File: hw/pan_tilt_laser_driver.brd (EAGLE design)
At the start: 76.2 x 34.2 mm, 38 parts, among them IC5 93C46, J1 POWER_JACKPTH, U1 CAT6219-330TDGT3, U3 LD3985M30R, X1 798-ZX62RD-AB-5P8, Y1 405I35D12M00000

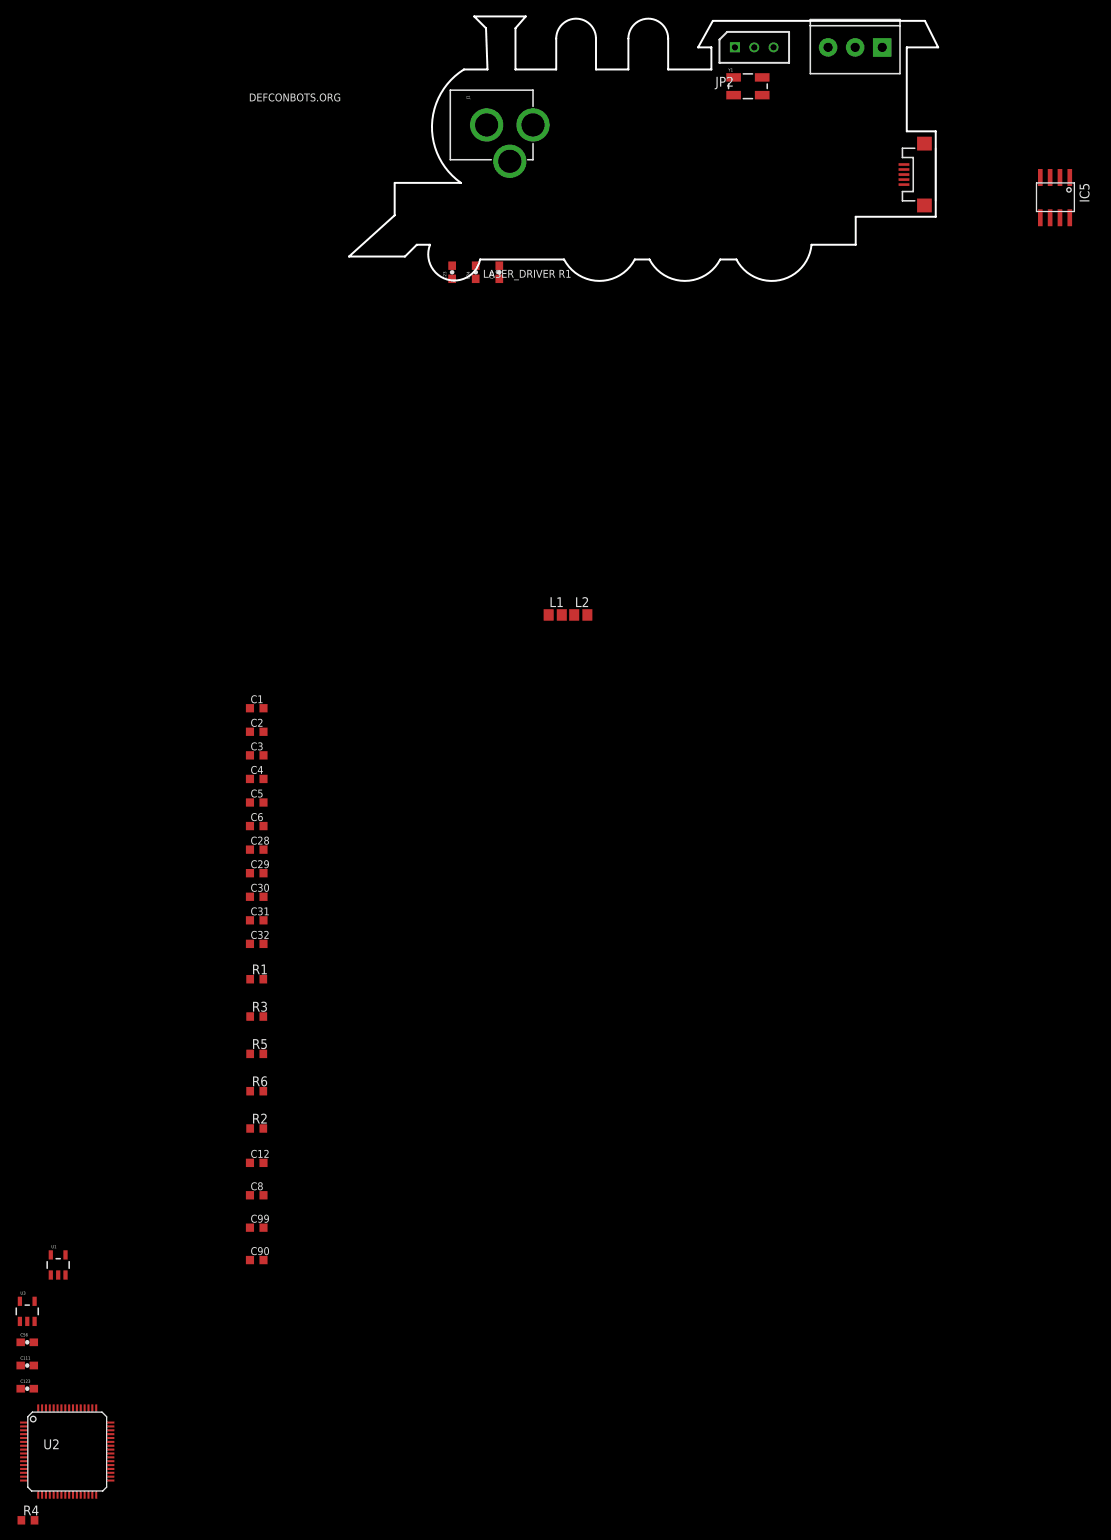
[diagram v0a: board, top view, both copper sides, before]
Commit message: Preliminary placement complete.
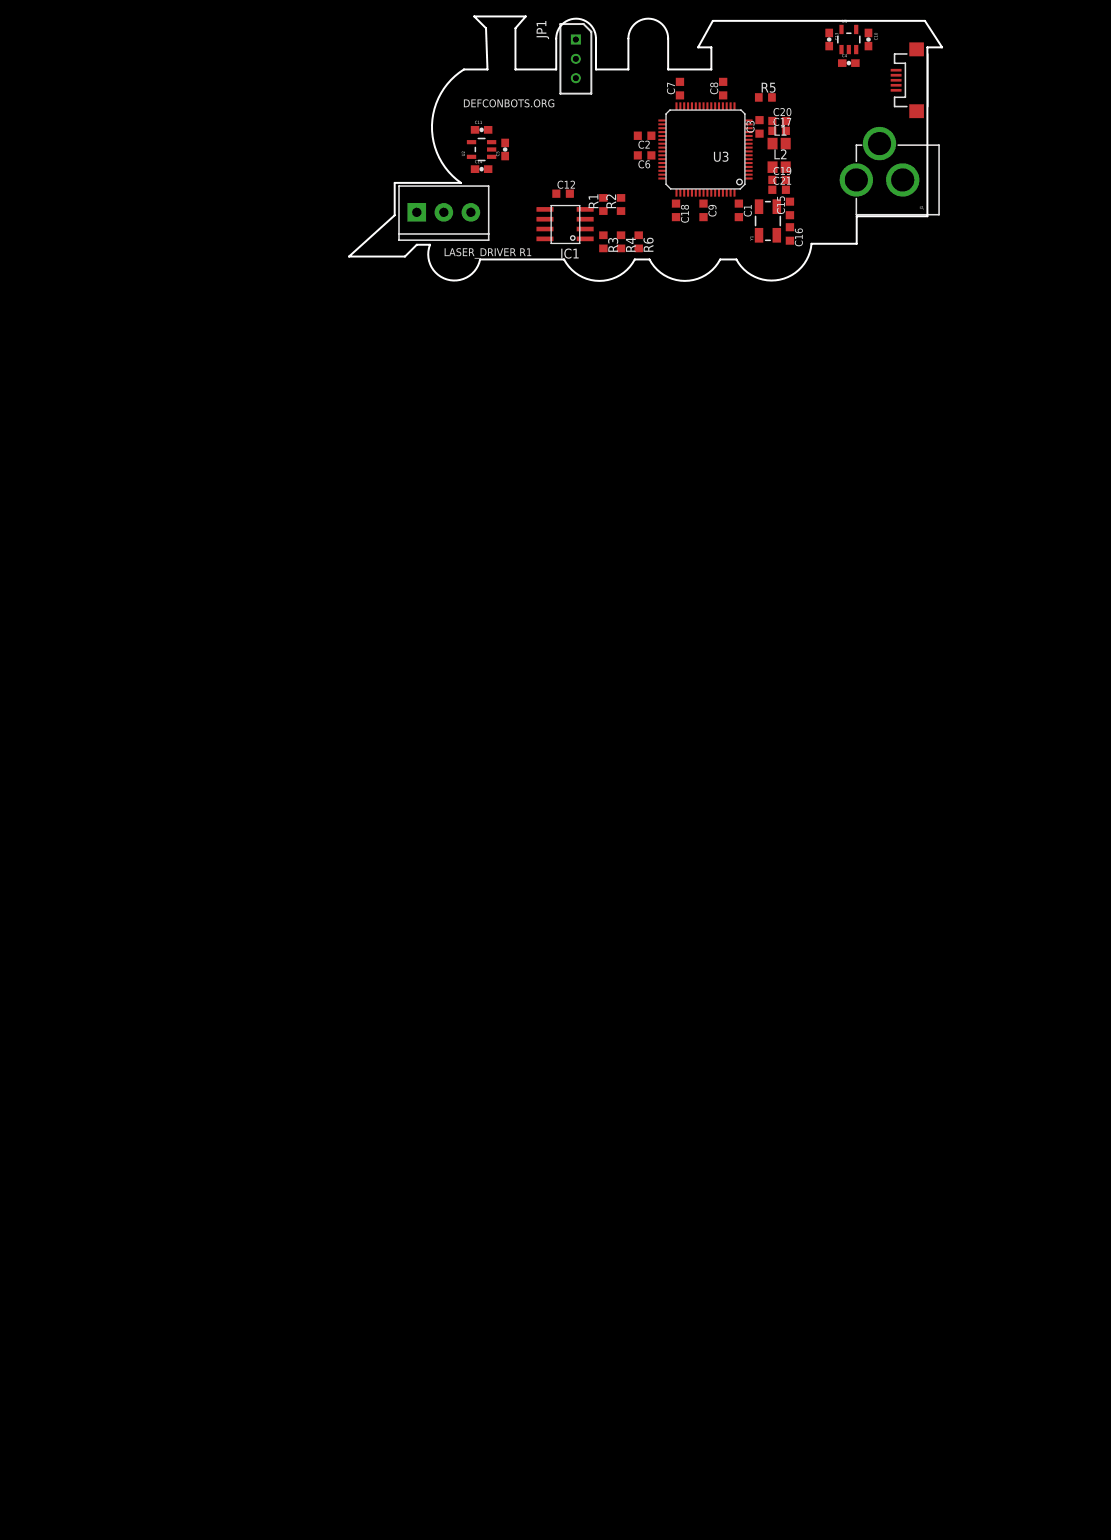
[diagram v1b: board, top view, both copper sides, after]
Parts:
- removed C111, C23, C24, C56: C1608X5R1C106M080AB, SparkFun-Passives:0603-CAP
- removed C123, C25: VJ0603A471KXQPW1BC, SparkFun-Passives:0603-CAP
- removed C28: (no value), rcl:C0603K
- removed C29, C30: 4.7u, rcl:C0603K
- removed C31, C32: 0.1u, rcl:C0603K
- removed C90, C99: 18p, rcl:C0603K
- removed IC5: 93C46, dp_devices:SOIC8
- added C10, C11: VJ0603A471KXQPW1BC, SparkFun-Passives:0603-CAP
- added C13, C14: C1608X5R1C106M080AB, SparkFun-Passives:0603-CAP
- added C15, C16: 18p, rcl:C0603K
- added C17, C19: 4.7u, rcl:C0603K
- added C18: 3.3u, rcl:C0603K
- added C20, C21: 0.1u, rcl:C0603K
- added C7, C9: (no value), rcl:C0603K
- added IC1: 93C46, dp_devices:SOIC8
- C12: value 3.3u -> .1u
- C4, C5: value (none) -> C1608X5R1C106M080AB; device rcl:C0603K -> SparkFun-Passives:0603-CAP
- C8: value .1u -> (none)
- JP1: value 651-5442251 -> (none); device SparkFun-Connectors:SCREWTERMINAL-3.5MM-3 -> torpedo:22-03-5035
- JP2: value (none) -> 651-5442251; device torpedo:22-03-5035 -> SparkFun-Connectors:SCREWTERMINAL-3.5MM-3
- R2: value 12k 1% -> 2.2k
- R4: value 2.2k -> 10k
- R5: value 10k -> 12k 1%
- U2: value (none) -> LD3985M30R; device torpedo:LQFP64 -> SparkFun-PowerIC:SOT23-5
- U3: value LD3985M30R -> (none); device SparkFun-PowerIC:SOT23-5 -> torpedo:LQFP64
- moved U1 188.6 mm to (64.3, 31.5)
- moved R4 182.3 mm to (34.8, 5.33), turned to 270 degrees
- moved U2 176.7 mm to (16.8, 17.3), turned to 90 degrees
- moved U3 174.0 mm to (45.7, 17.3), turned to 180 degrees
- moved C8 155.3 mm to (48.0, 25.1), turned to 90 degrees
- moved R5 140.1 mm to (53.5, 24.0)
- moved C12 131.5 mm to (27.3, 11.6)
- moved R2 128.5 mm to (34.8, 10.2), turned to 90 degrees
- moved R6 120.5 mm to (37.1, 5.33), turned to 270 degrees
- moved C4 120.2 mm to (64.3, 28.4)
- moved R1 109.8 mm to (32.5, 10.2), turned to 90 degrees
- moved R3 109.8 mm to (32.5, 5.33), turned to 270 degrees
- moved C3 104.1 mm to (52.7, 20.2), turned to 90 degrees
- moved C6 100.2 mm to (37.8, 16.5), turned to 180 degrees
- moved C2 92.0 mm to (37.8, 19.1), turned to 180 degrees
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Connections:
- net !RESET: now also U3.14; no longer U2.14
- net 1.8V: now also C18.1, U3.12, U3.37, U3.49, U3.64; no longer C12.1, U2.12, U2.37, U2.49, U2.64
- net 3.3V: now also C12.1, C13.1, C7.1, C9.1, IC1.6, IC1.8, R4.2, U3.20, U3.31, U3.42, U3.50, U3.56; no longer C24.1, C28.1, C4.1, C5.1, IC5.6, IC5.8, R5.2, U2.20, U2.31, U2.42, U2.50, U2.56
- net 5V: now also C4.1, C5.1, U2.1; no longer C23.1, C56.1, U3.1
- net EECLK: now also IC1.2, R4.1, U3.62; no longer IC5.2, R5.1, U2.62
- net EECS: now also IC1.1, U3.63; no longer IC5.1, U2.63
- net EEDATA: now also IC1.3, R2.1, U3.61; no longer IC5.3, R4.1, U2.61
- net GND: now also C10.2, C11.2, C13.2, C14.2, C15.1, C16.1, C17.2, C18.2, C19.2, C20.2, C21.2, C7.2, C9.2, IC1.5, JP1.1, JP2.3, R5.2, U2.2, U3.1, U3.10, U3.11, U3.13, U3.15, U3.25, U3.35, U3.47, U3.5, U3.51; no longer C111.2, C123.2, C23.2, C24.2, C25.2, C28.2, C29.2, C30.2, C31.2, C32.2, C56.2, C90.1, C99.1, IC5.5, JP1.3, JP2.1, R2.2, U2.1, U2.10, U2.11, U2.13, U2.15, U2.25, U2.35, U2.47, U2.5, U2.51, U3.2
- net LASER_EN: now also U2.3, U3.21; no longer U2.21, U3.3
- net LASER_PWR: now also C14.1, JP2.1, U2.5; no longer C111.1, JP1.1, U3.5
- net LASER_TXD: now also JP2.2, U3.16; no longer JP1.2, U2.16
- net N$1: now also C11.1, U2.4; no longer C123.1, U3.4
- net N$10: now also C16.2, U3.3; no longer C90.2, U2.3
- net N$3: now also U3.7; no longer U2.7
- net N$4: now also R5.1, U3.6; no longer R2.1, U2.6
- net N$45: now also IC1.4, R2.2; no longer IC5.4, R4.2
- net N$5: now also U3.8; no longer U2.8
- net N$6: now also C17.1, C20.1, U3.9; no longer C29.1, C31.1, U2.9
- net N$7: now also C15.2, U3.2; no longer C99.2, U2.2
- net N$8: now also C10.1; no longer C25.1
- net N$9: now also C19.1, C21.1, U3.4; no longer C30.1, C32.1, U2.4
- net PAN_TILT_TXD: now also JP1.3, U3.38; no longer JP2.3, U2.38
- net SERVO_POWER: now also JP1.2; no longer JP2.2
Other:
- board size 76.2 x 34.2 mm -> 76.7 x 34.2 mm
